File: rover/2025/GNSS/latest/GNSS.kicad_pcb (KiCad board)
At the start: 4 copper layers, 50 x 50 mm, 42 parts, among them J1 Eth-Horiz, J2 Eth-Horiz, J4 JST6_Pin, J5 USB_C_USB4145-GCT, SW1 TS09-63-25-WT-160-SMT-TR, SW2 TS09-63-25-WT-160-SMT-TR, U1 SN65HVD232, U2 ESP32-S3-WROVER, U3 Volt_check-NCV308, U4 LDO-TLV74033PDBVR, U5 TVS, U6 DC_DC-AP64501

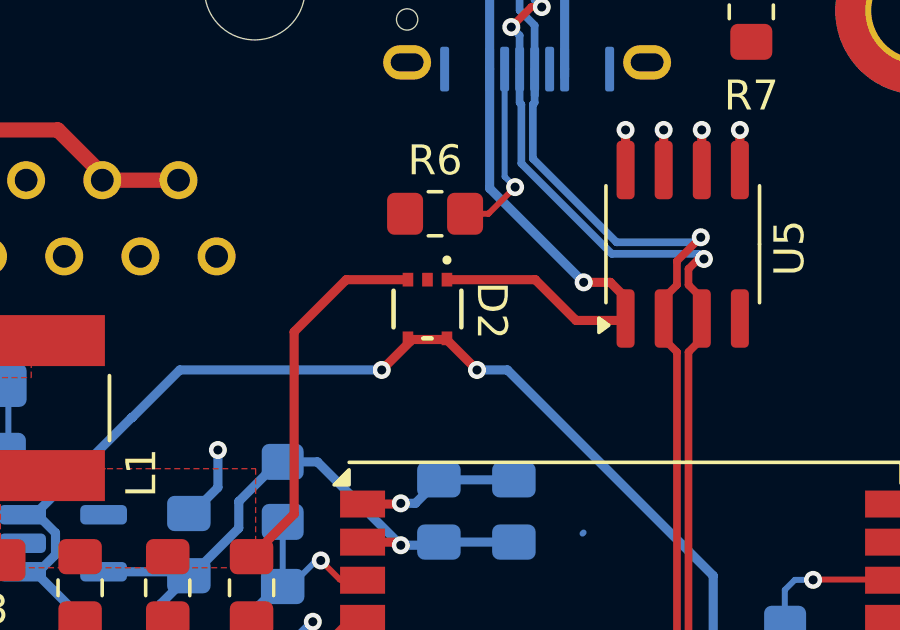
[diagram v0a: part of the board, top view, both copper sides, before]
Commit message: footprint update
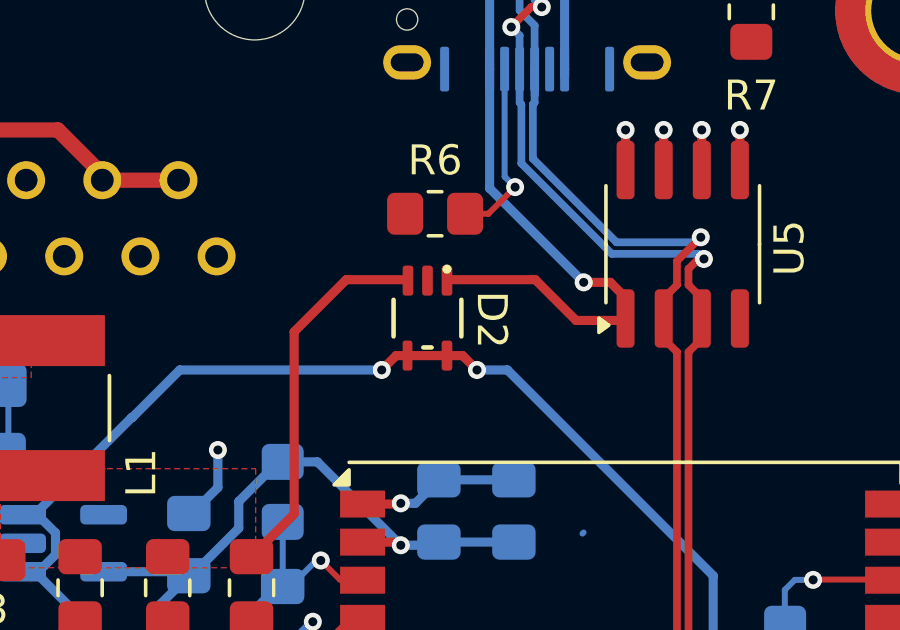
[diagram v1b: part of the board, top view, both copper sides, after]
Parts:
- moved D2 0.30 mm to (157.6, 84.2)
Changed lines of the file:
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@@
 	(footprint "RoverFootprint:Diode_schottky-CVJ10F30"
 		(layer "F.Cu")
-		(at 157.607 83.947 -90)
+		(at 157.607 84.25 -90)
 		(tags "CVJ10F30_LF ")
 		(property "Reference" "D2"
@@
 			)
 		)
-		(property "Status" "TO BE VERIFIED"
-			(at 0 0 270)
-			(unlocked yes)
-			(layer "F.Fab")
-			(hide yes)
-			(effects
-				(font
-					(size 1 1)
-					(thickness 0.15)
-				)
-			)
-		)
 		(sheetname "/")
 		(sheetfile "GNSS.kicad_sch")
@@
 			)
 		)
-		(pad "1" smd rect
-			(at -0.9779 -0.649999 270)
-			(size 0.4572 0.3556)
+		(pad "1" smd roundrect
+			(at -1.24965 -0.649999 270)
+			(size 1.0007 0.3556)
 			(layers "F.Cu" "F.Mask" "F.Paste")
+			(roundrect_rratio 0.25)
 			(net 14 "+5V_USB")
 			(pintype "passive")
 		)
-		(pad "2" smd rect
-			(at -0.9779 0 270)
-			(size 0.4572 0.3556)
+		(pad "2" smd roundrect
+			(at -1.24965 0 270)
+			(size 1.0007 0.3556)
 			(layers "F.Cu" "F.Mask" "F.Paste")
+			(roundrect_rratio 0.25)
 			(net 64 "unconnected-(D2-NC-Pad2)")
 			(pinfunction "NC")
 			(pintype "passive")
 		)
-		(pad "3" smd rect
-			(at -0.9779 0.649999 270)
-			(size 0.4572 0.3556)
+		(pad "3" smd roundrect
+			(at -1.24965 0.649999 270)
+			(size 1.0007 0.3556)
 			(layers "F.Cu" "F.Mask" "F.Paste")
+			(roundrect_rratio 0.25)
 			(net 56 "+5V_ETH")
 			(pintype "passive")
 		)
-		(pad "4" smd rect
-			(at 0.9779 0.649999 270)
-			(size 0.4572 0.3556)
+		(pad "4" smd roundrect
+			(at 1.24965 0.663899 270)
+			(size 1.0007 0.327798)
 			(layers "F.Cu" "F.Mask" "F.Paste")
+			(roundrect_rratio 0.25)
 			(net 3 "+5V")
 			(pintype "passive")
 		)
-		(pad "5" smd rect
-			(at 0.9779 -0.649999 270)
-			(size 0.4572 0.3556)
+		(pad "5" smd roundrect
+			(at 1.24965 -0.649999 270)
+			(size 1.0007 0.3556)
 			(layers "F.Cu" "F.Mask" "F.Paste")
+			(roundrect_rratio 0.25)
 			(net 3 "+5V")
 			(pintype "passive")
@@
 			(keep_text_aligned yes)
 		)
-		(gr_text "1968.5039 mils"
+		(gr_text "50.0000 mm"
 			(at 153 130.675999 0)
 			(layer "User.1")
@@
 			(keep_text_aligned yes)
 		)
-		(gr_text "1653.5433 mils"
+		(gr_text "42.0000 mm"
 			(at 182.111 95 90)
 			(layer "User.1")
@@
 			(keep_text_aligned yes)
 		)
-		(gr_text "1968.5039 mils"
+		(gr_text "50.0000 mm"
 			(at 185.667 95 90)
 			(layer "User.1")
@@
 	)
 	(segment
-		(start 158.242 84.963)
-		(end 157.099 84.963)
+		(start 159.258 85.979)
+		(end 158.779 85.5)
 		(width 0.3048)
 		(layer "F.Cu")
@@
 	)
 	(segment
-		(start 157.099 84.963)
+		(start 156.562 85.5)
 		(end 156.083 85.979)
 		(width 0.3048)
@@
 	)
 	(segment
-		(start 159.258 85.979)
-		(end 158.242 84.963)
+		(start 158.779 85.5)
+		(end 156.562 85.5)
 		(width 0.3048)
 		(layer "F.Cu")
